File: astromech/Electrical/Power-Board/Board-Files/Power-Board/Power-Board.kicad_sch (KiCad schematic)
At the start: 72 parts, among them J1 BAT_IN_SCREW, J10 HEAD_MOT, J2 BAT_IN_HOLE, J5 E_STOP, J6 CTRL_BRD, J7 JETSON, J8 L_DRIVE, J9 R_DRIVE, Q1 Q_NMOS_DSG, Q2 Q_NMOS_DSG, U1 LTC7003, U2 Logic_Level_Converter, U3 D36V50Fx, U4 LTC7003, U5 D36V50Fx, U6 D36V50Fx

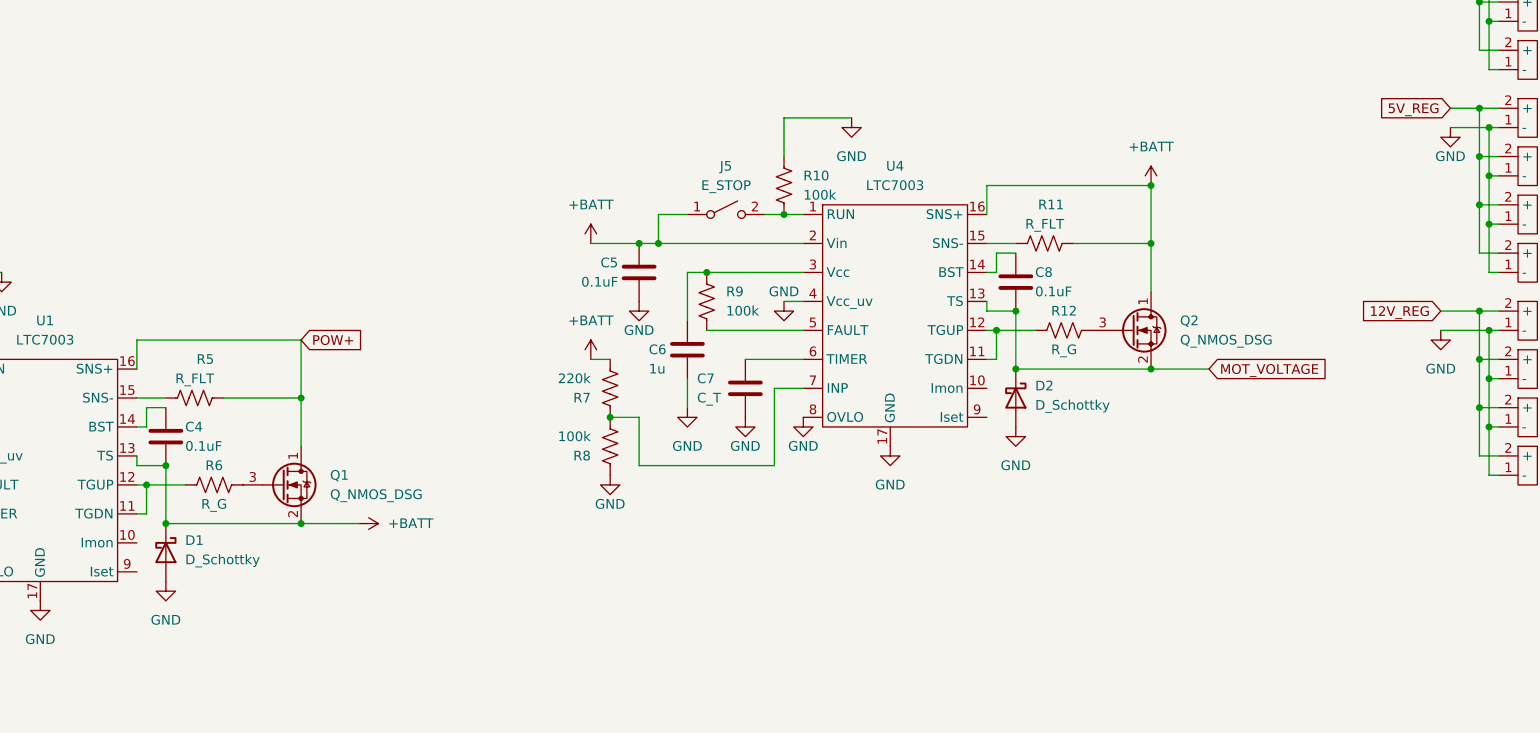
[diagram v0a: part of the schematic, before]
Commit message: added test points
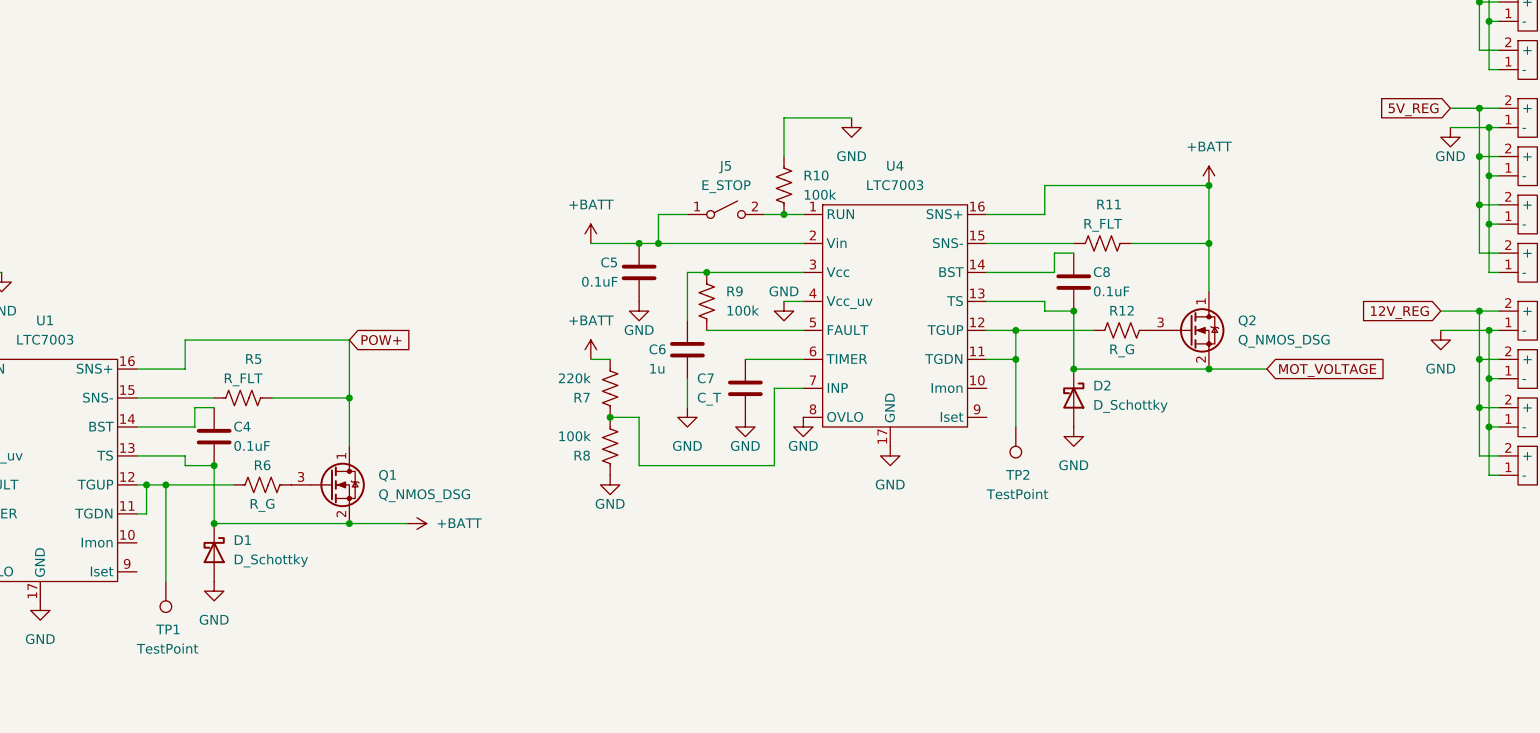
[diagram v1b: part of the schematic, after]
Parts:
- added TP1, TP2: TestPoint, symbol Connector:TestPoint
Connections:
- net at R12.1, U4.11 (TGDN), U4.12 (TGUP): now also TP2.1
- net at R6.1, U1.11 (TGDN), U1.12 (TGUP): now also TP1.1
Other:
- moved on the sheet: C4, C8, D1, D2, Q1, Q2, R11, R12, R5, R6
